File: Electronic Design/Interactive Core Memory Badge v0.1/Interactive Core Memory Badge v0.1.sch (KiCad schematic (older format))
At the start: 7 parts, among them Q1 MMBT4403LT1G, Q2 MMBT4401LT1G

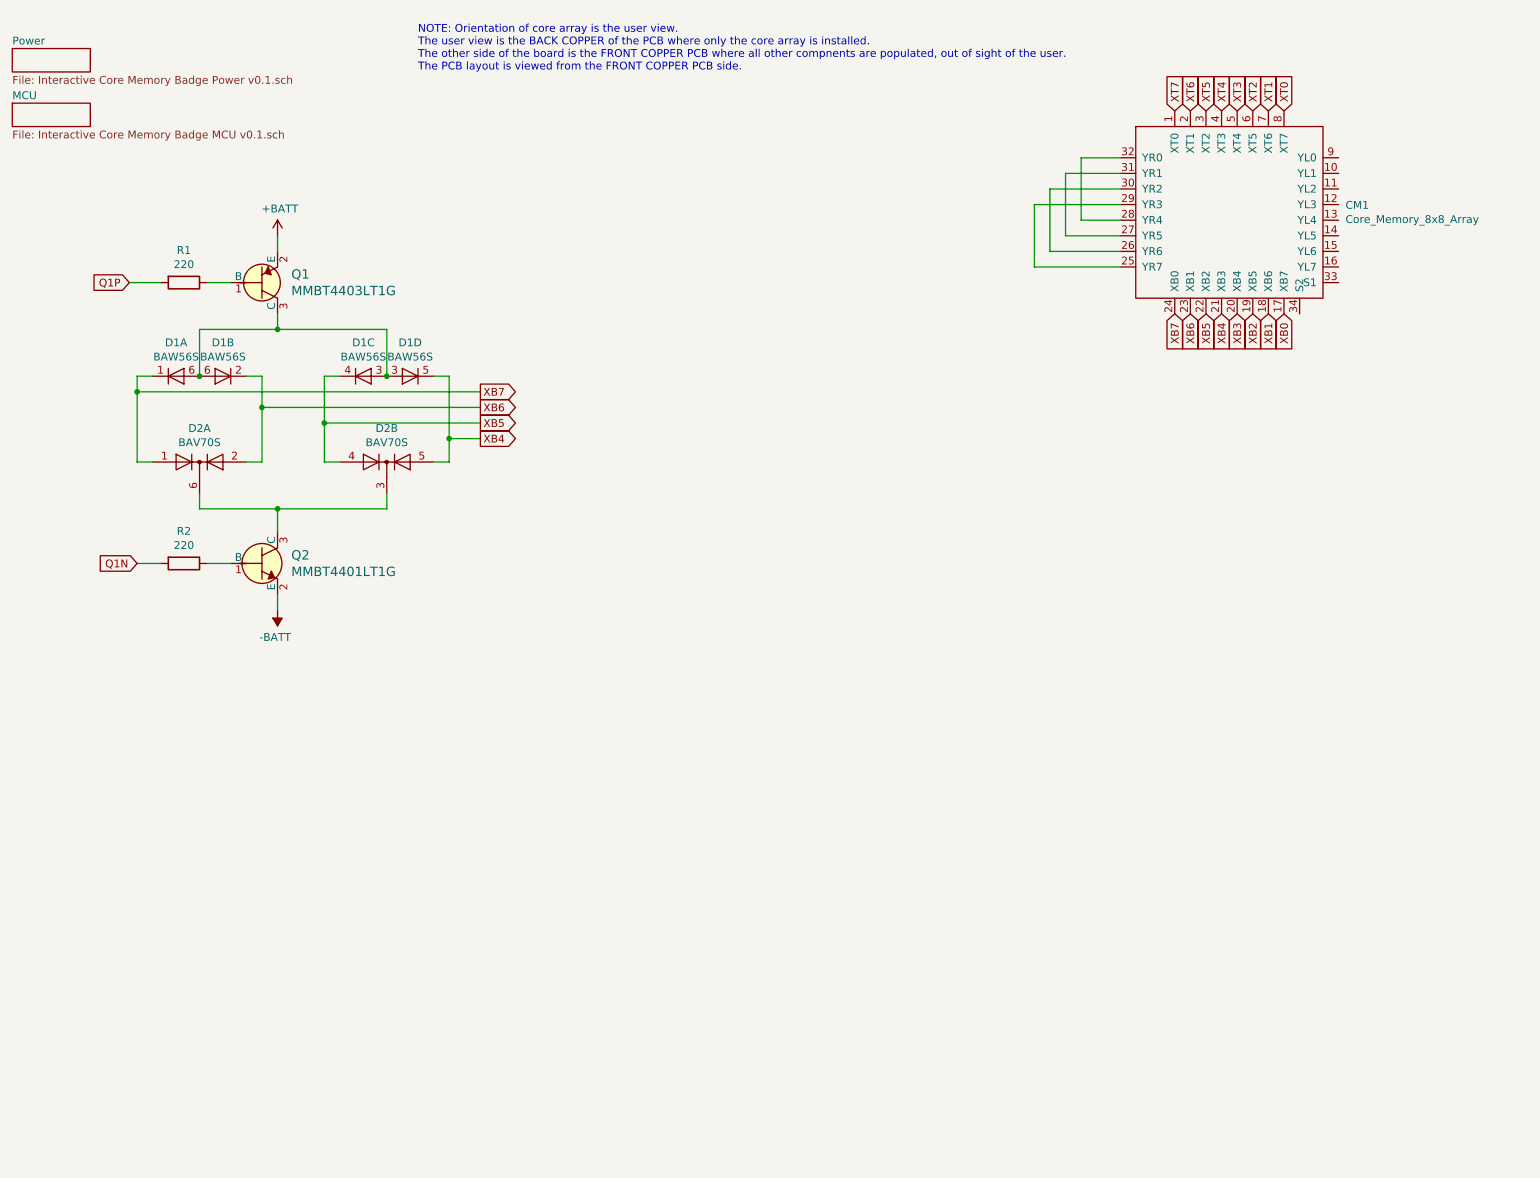
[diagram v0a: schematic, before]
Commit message: Schematic Complete
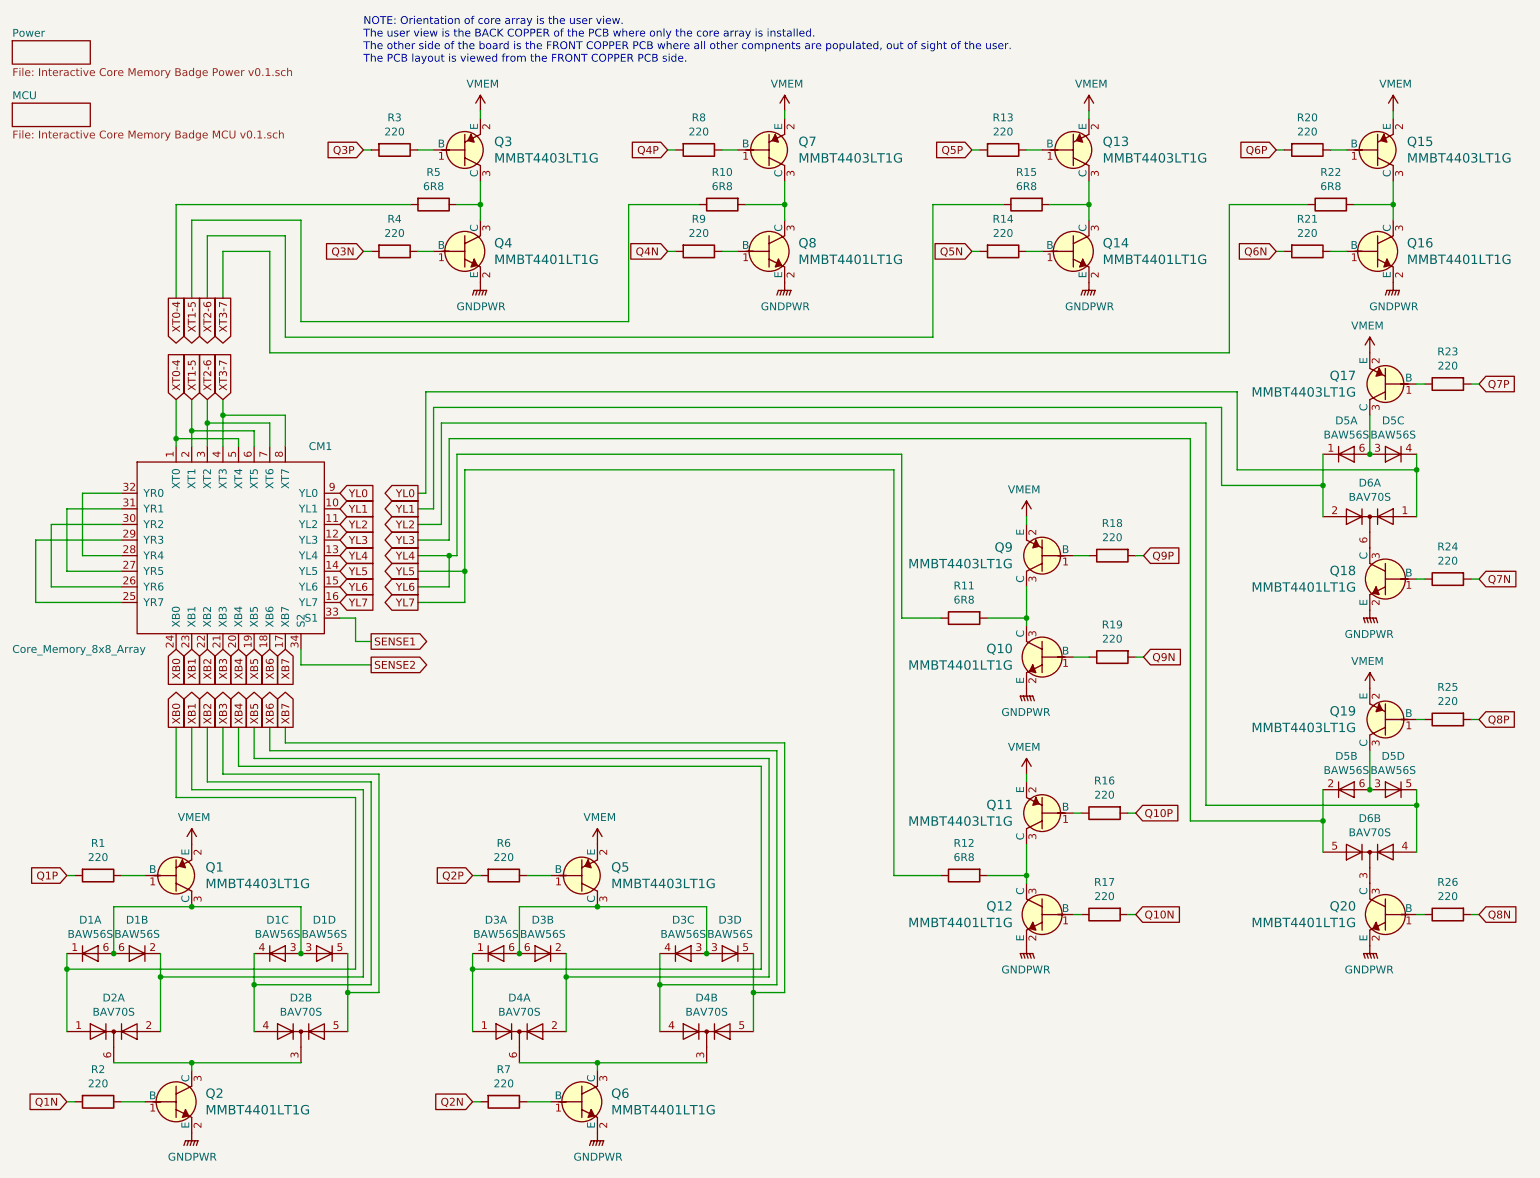
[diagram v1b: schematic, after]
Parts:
- added D3, D5: BAW56S, Package_TO_SOT_SMD:SOT-363_SC-70-6, symbol Diode:BAW56S
- added D4, D6: BAV70S, Package_TO_SOT_SMD:SOT-363_SC-70-6, symbol Diode:BAV70S
- added Q10, Q12, Q14, Q16, Q18, Q20, Q4, Q6, Q8: MMBT4401LT1G, Digikey:SOT-23-3, symbol Digikey-Transistors:MMBT4401LT1G
- added Q11, Q13, Q15, Q17, Q19, Q3, Q5, Q7, Q9: MMBT4403LT1G, Digikey:SOT-23-3, symbol Digikey-Transistors:MMBT4403LT1G
- added R10, R11, R12, R15, R22, R5: 6R8, Resistor_SMD:R_0805_2012Metric, symbol Device:R
- added R13, R14, R16, R17, R18, R19, R20, R21, R23, R24, R25, R26, R3, R4, R6, R7, R8, R9: 220, Resistor_SMD:R_0805_2012Metric, symbol Device:R
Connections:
- net XT4 is gone; now on net XT3-7: CM1.4 (XT3)
- net XT5 is gone; now on net XT2-6: CM1.3 (XT2)
- net XT6 is gone; now on net XT1-5: CM1.2 (XT1)
- net XT7 is gone; now on net XT0-4: CM1.1 (XT0)
- net XB0: now also CM1.24 (XB0), D1.1 (K), D2.1 (A); no longer CM1.17 (XB7)
- net XB1: now also CM1.23 (XB1), D1.2 (K), D2.2 (A); no longer CM1.18 (XB6)
- net XB2: now also CM1.22 (XB2), D1.4 (K), D2.4 (A); no longer CM1.19 (XB5)
- net XB3: now also CM1.21 (XB3), D1.5 (K), D2.5 (A); no longer CM1.20 (XB4)
- net XB4: now also CM1.20 (XB4), D3.1 (K), D4.1 (A); no longer CM1.21 (XB3), D1.5 (K), D2.5 (A)
- net XB5: now also CM1.19 (XB5), D3.2 (K), D4.2 (A); no longer CM1.22 (XB2), D1.4 (K), D2.4 (A)
- net XB6: now also CM1.18 (XB6), D3.4 (K), D4.4 (A); no longer CM1.23 (XB1), D1.2 (K), D2.2 (A)
- net XB7: now also CM1.17 (XB7), D3.5 (K), D4.5 (A); no longer CM1.24 (XB0), D1.1 (K), D2.1 (A)
- net YL1: now reaches CM1.10 (YL1)
- net YL1: now also D5.1 (K), D6.2 (A)
- net YL2: now reaches CM1.11 (YL2)
- net YL2: now also D5.5 (K), D6.4 (A)
- net YL3: now reaches CM1.12 (YL3)
- net YL3: now also D5.2 (K), D6.5 (A)
- net YL4: now reaches CM1.13 (YL4)
- net YL4: now also CM1.15 (YL6), R11.1
- net YL5: now reaches CM1.14 (YL5)
- net YL5: now also CM1.16 (YL7), R12.1
- net SENSE1: now reaches CM1.33 (S1)
- net SENSE2: now reaches CM1.34 (S2)
- net YL0: now reaches CM1.9 (YL0)
- net YL0: now also D5.4 (K), D6.1 (A)
- net +BATT renamed VMEM
- net VMEM: now also Q11.2 (E), Q13.2 (E), Q15.2 (E), Q17.2 (E), Q19.2 (E), Q3.2 (E), Q5.2 (E), Q7.2 (E), Q9.2 (E)
- net -BATT renamed GNDPWR
- net GNDPWR: now also Q10.2 (E), Q12.2 (E), Q14.2 (E), Q16.2 (E), Q18.2 (E), Q20.2 (E), Q4.2 (E), Q6.2 (E), Q8.2 (E)
- net XT0 renamed XT3-7
- net XT3-7: now also R22.1
- net XT1 renamed XT2-6
- net XT2-6: now also R15.1
- net XT2 renamed XT1-5
- net XT1-5: now also R10.1
- net XT3 renamed XT0-4
- net XT0-4: now also R5.2
- new net: Q4.1 (B), R4.1
- new net: Q3.1 (B), R3.1
- new net: Q3.3 (C), Q4.3 (C), R5.1
- new net: D5.3 (A), D5.6 (A), Q17.3 (C)
- new net: Q17.1 (B), R23.1
- new net: Q18.1 (B), R24.1
- new net: D6.6 (K), Q18.3 (C)
- new net: D3.3 (A), D3.3 (A), D3.6 (A), D3.6 (A), Q5.3 (C)
- new net: Q5.1 (B), R6.1
- new net: Q6.1 (B), R7.1
- new net: D4.3 (K), D4.6 (K), Q6.3 (C)
- new net: D5.3 (A), D5.6 (A), Q19.3 (C)
- new net: Q19.1 (B), R25.1
- new net: Q20.1 (B), R26.1
- new net: D6.3 (K), Q20.3 (C)
- new net: Q7.1 (B), R8.1
- new net: Q7.3 (C), Q8.3 (C), R10.2
- new net: Q8.1 (B), R9.1
- new net: Q13.1 (B), R13.1
- new net: Q13.3 (C), Q14.3 (C), R15.2
- new net: Q14.1 (B), R14.1
- new net: Q15.1 (B), R20.1
- new net: Q15.3 (C), Q16.3 (C), R22.2
- new net: Q16.1 (B), R21.1
- new net: Q9.1 (B), R18.1
- new net: Q10.3 (C), Q9.3 (C), R11.2
- new net: Q10.1 (B), R19.1
- new net: Q11.1 (B), R16.1
- new net: Q11.3 (C), Q12.3 (C), R12.2
- new net: Q12.1 (B), R17.1
- new net Q10N: R17.2
- new net Q10P: R16.2
- new net Q2N: R7.2
- new net Q2P: R6.2
- new net Q3N: R4.2
- new net Q3P: R3.2
- new net Q4N: R9.2
- new net Q4P: R8.2
- new net Q5N: R14.2
- new net Q5P: R13.2
- new net Q6N: R21.2
- new net Q6P: R20.2
- new net Q7N: R24.2
- new net Q7P: R23.2
- new net Q8N: R26.2
- new net Q8P: R25.2
- new net Q9N: R19.2
- new net Q9P: R18.2
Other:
- moved on the sheet: CM1
